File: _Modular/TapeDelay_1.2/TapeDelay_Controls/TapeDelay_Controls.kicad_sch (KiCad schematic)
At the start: 27 parts, among them J1 Interrupt, J3 Encoder/Enter/ESC, J4 OLED, J5 CPU I2C, SW1 Unload, SW2 Run/Pause, SW3 RotaryEncoder_Switch, SW4 Escape, U1 PCF8574

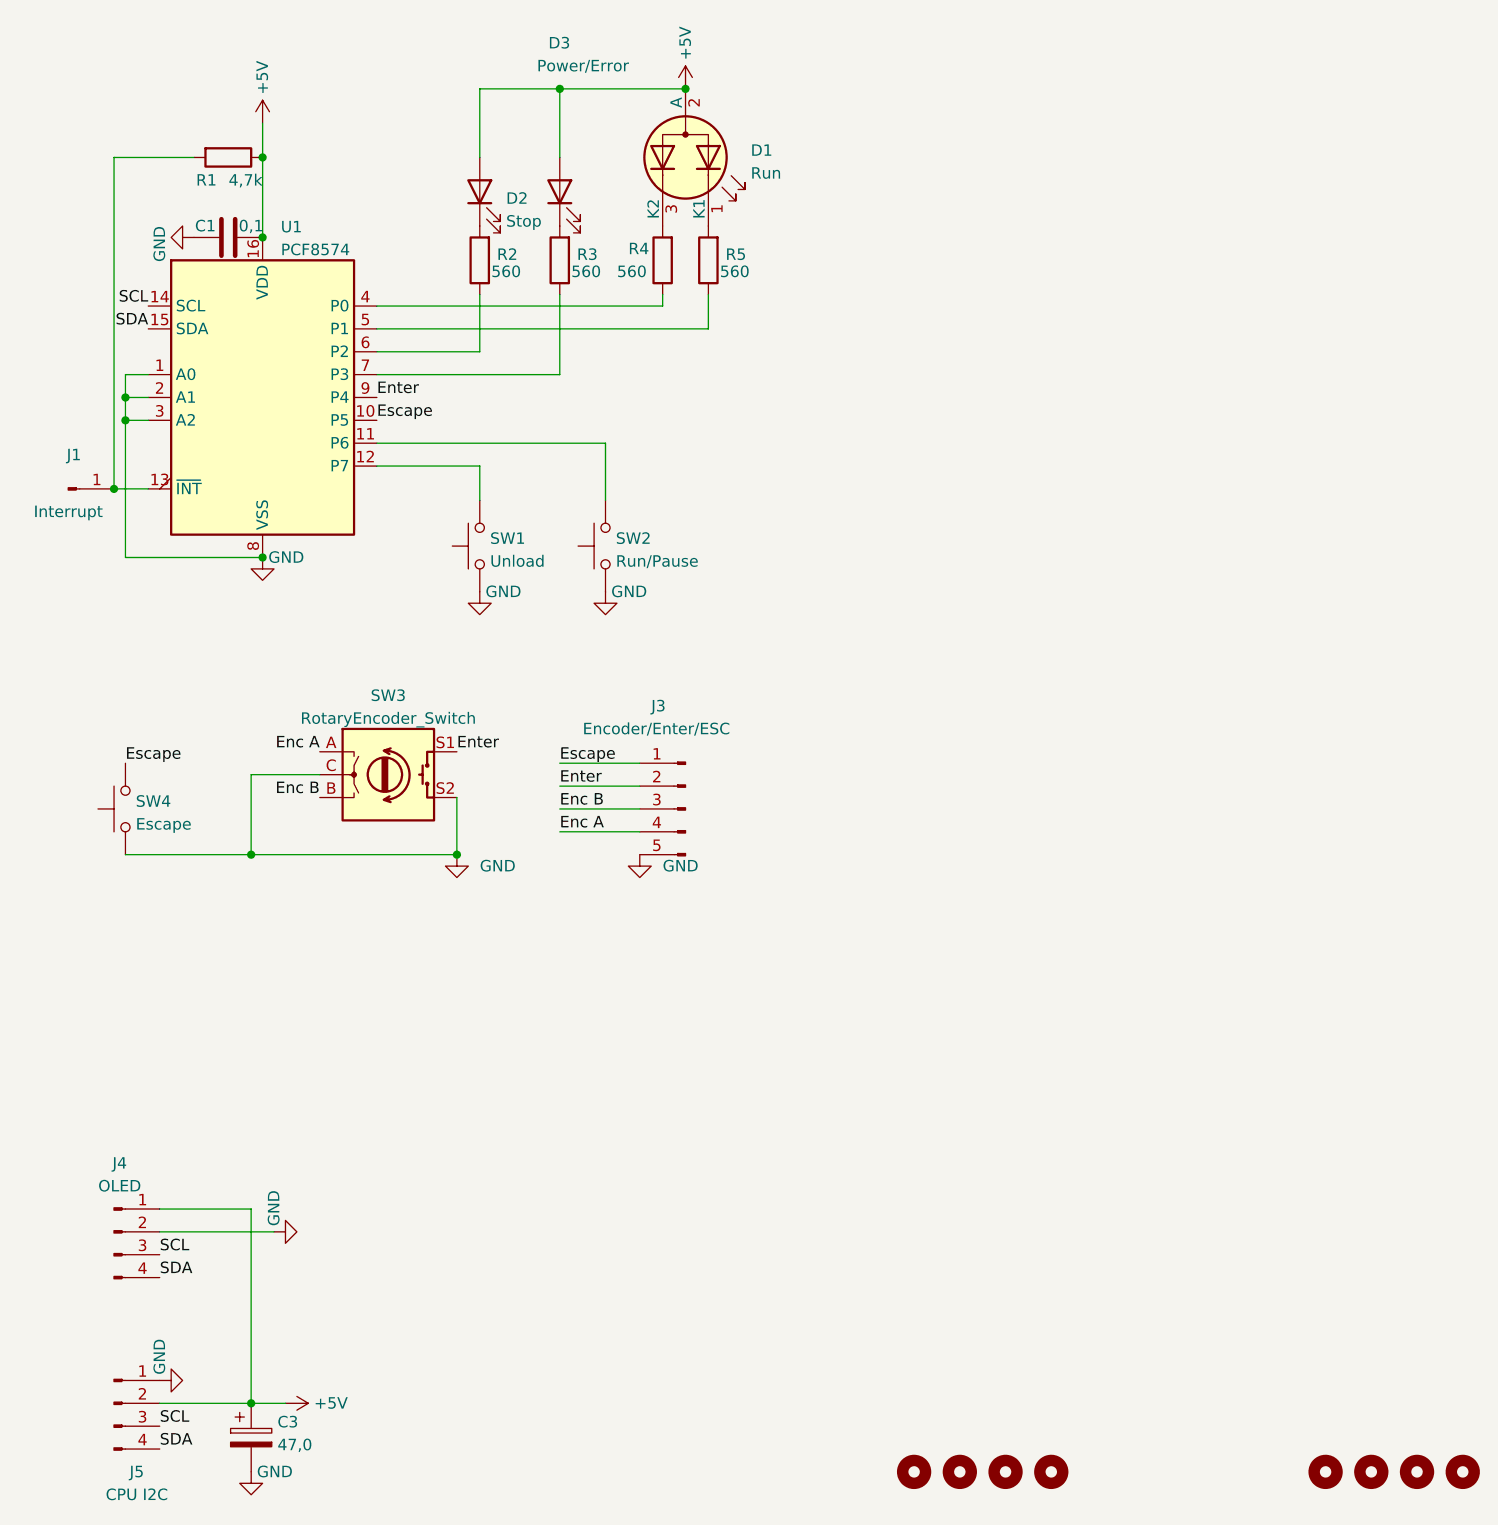
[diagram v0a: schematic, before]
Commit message: up
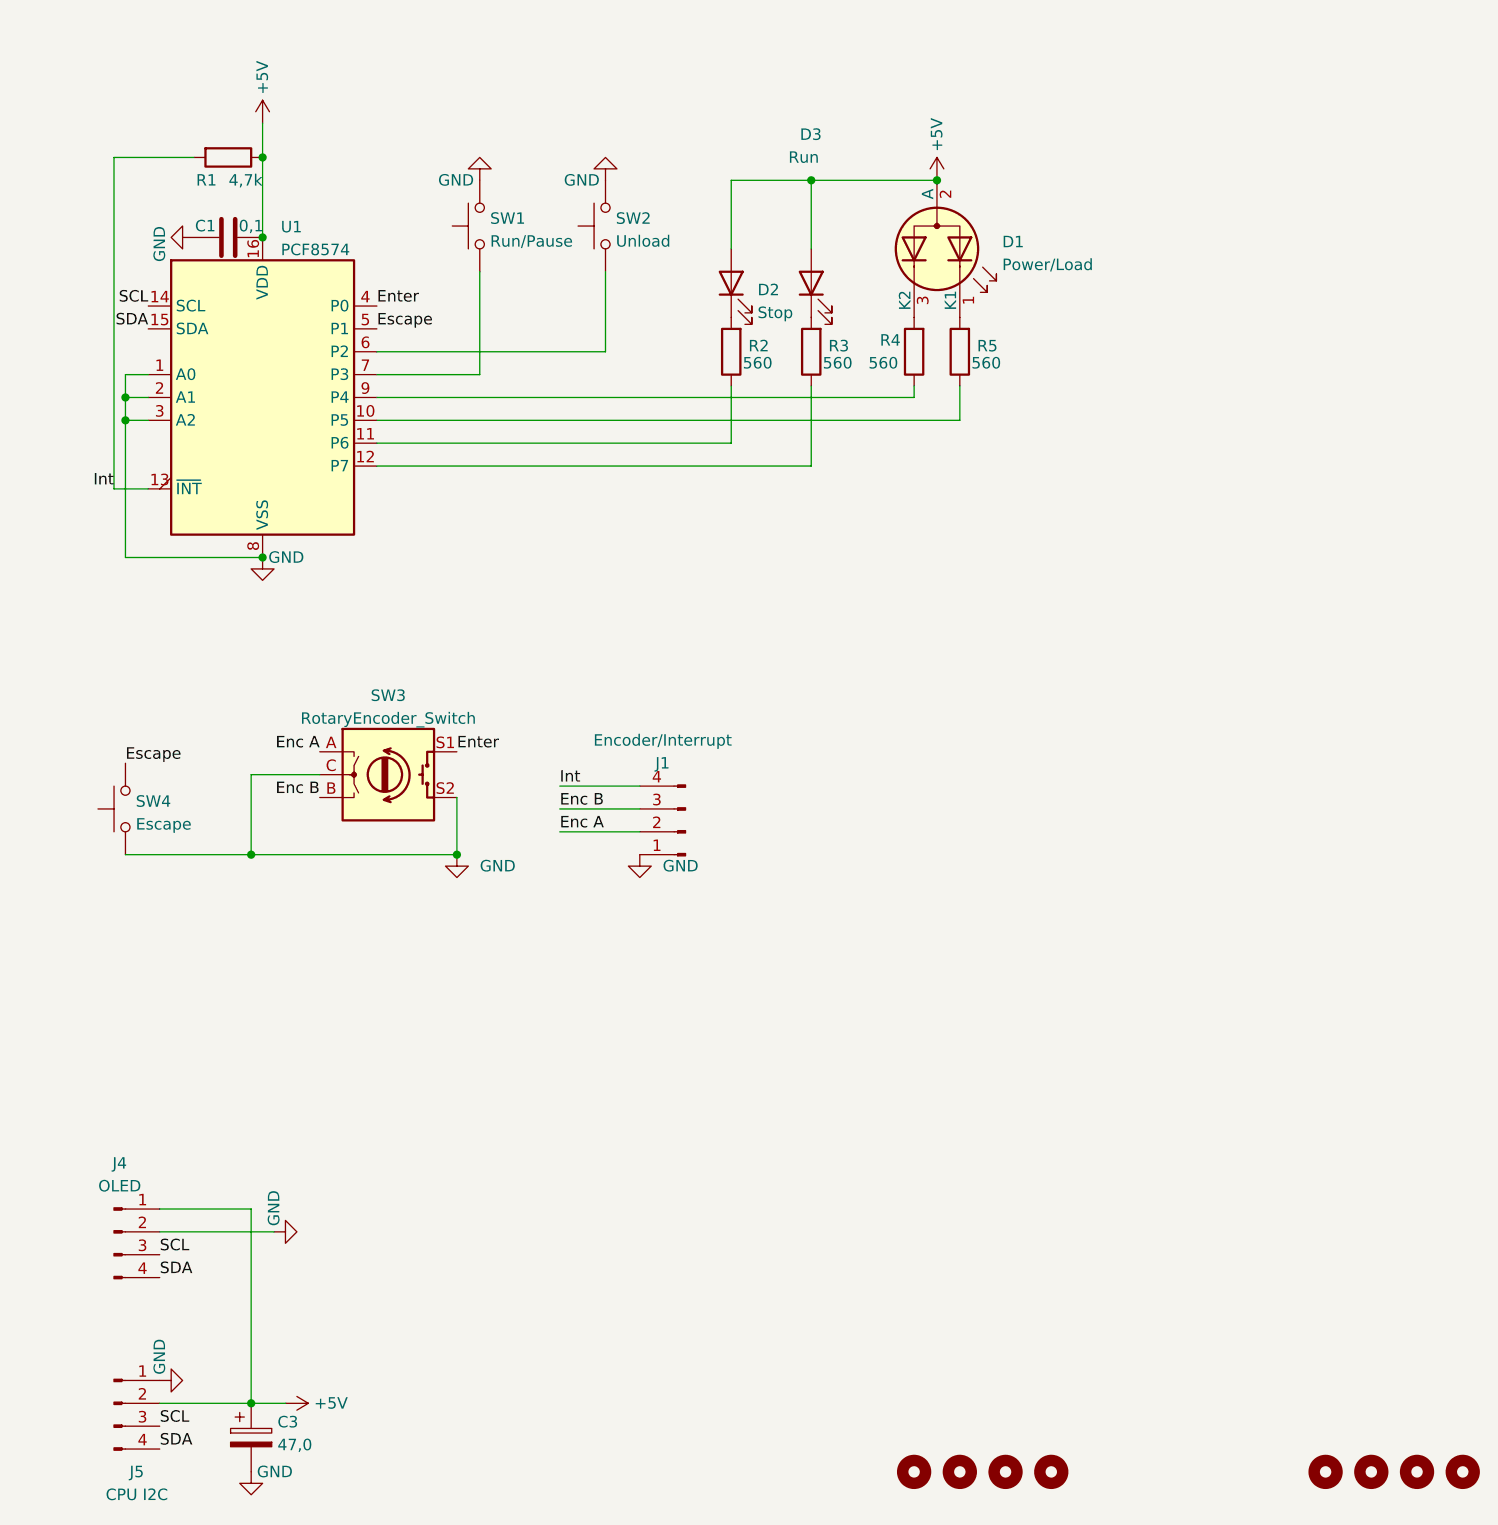
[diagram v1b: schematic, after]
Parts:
- removed J1: Interrupt, Connector_PinHeader_2.54mm:PinHeader_1x01_P2.54mm_Vertical, symbol Connector:Conn_01x01_Male
- removed J3: Encoder/Enter/ESC, Connector_PinHeader_2.54mm:PinHeader_1x05_P2.54mm_Vertical, symbol Connector:Conn_01x05_Male
- added J1: Encoder/Interrupt, Connector_PinHeader_2.54mm:PinHeader_1x04_P2.54mm_Vertical, symbol Connector:Conn_01x04_Male
- D1: value Run -> Power/Load
- D3: value Power/Error -> Run
- SW1: value Unload -> Run/Pause
- SW2: value Run/Pause -> Unload
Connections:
- net Enc A: now also J1.2 (Pin_2)
- net Enc B: now also J1.3 (Pin_3)
- net Enter: now also U1.4 (P0); no longer U1.9 (P4)
- net Escape: now also U1.5 (P1); no longer U1.10 (P5)
- net GND: now also J1.1 (Pin_1)
- net Int: now reaches R1.2, U1.13 (~{INT})
- net Int: now also J1.4 (Pin_4)
- net at R3.1: now also U1.12 (P7); no longer U1.7 (P3)
- net at R4.1: now also U1.9 (P4); no longer U1.4 (P0)
- net at SW1.2: now also U1.7 (P3); no longer U1.12 (P7)
- net at SW2.2: now also U1.6 (P2); no longer U1.11 (P6)
- net at R2.1: now also U1.11 (P6); no longer U1.6 (P2)
- net at R5.1: now also U1.10 (P5); no longer U1.5 (P1)
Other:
- moved on the sheet: D1, D2, D3, R2, R3, R4, R5, SW1, SW2

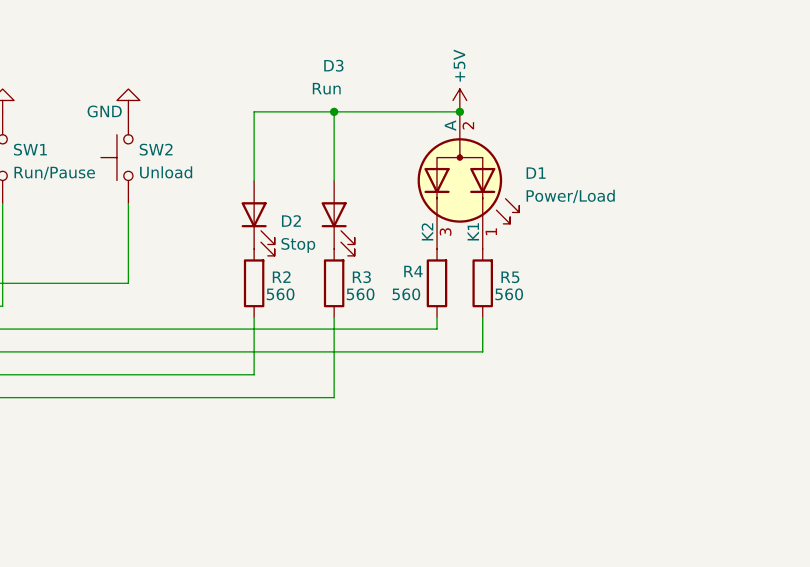
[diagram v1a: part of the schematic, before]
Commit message: up
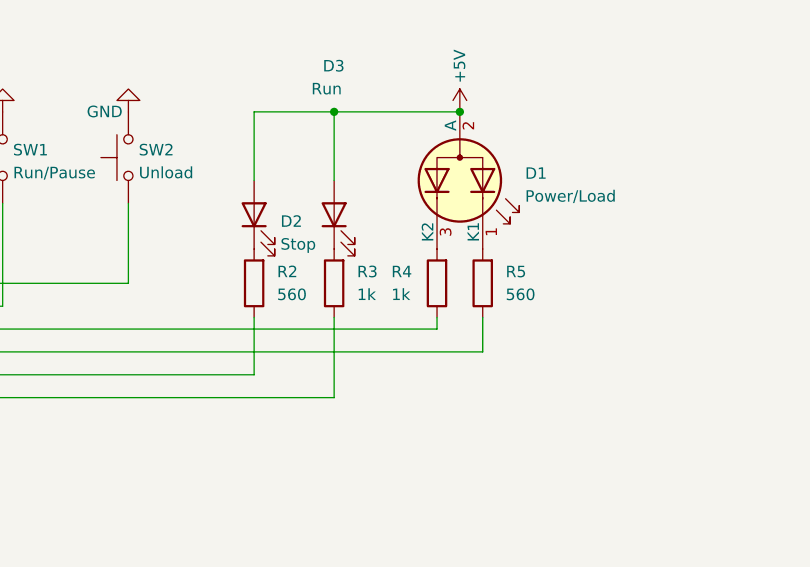
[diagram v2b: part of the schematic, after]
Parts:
- R3, R4: value 560 -> 1k
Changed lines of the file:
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@@
   (symbol (lib_id "Device:R") (at 99.06 67.31 180) (unit 1)
     (in_bom yes) (on_board yes)
-    (property "Reference" "R3" (id 0) (at 100.965 66.675 0)
-      (effects (font (size 1.27 1.27)) (justify right))
-    )
-    (property "Value" "560" (id 1) (at 100.33 68.58 0)
+    (property "Reference" "R3" (id 0) (at 101.6 66.04 0)
+      (effects (font (size 1.27 1.27)) (justify right))
+    )
+    (property "Value" "1k" (id 1) (at 101.6 68.58 0)
       (effects (font (size 1.27 1.27)) (justify right))
     )
@@
   (symbol (lib_id "Device:R") (at 110.49 67.31 180) (unit 1)
     (in_bom yes) (on_board yes)
-    (property "Reference" "R4" (id 0) (at 106.68 66.04 0)
-      (effects (font (size 1.27 1.27)) (justify right))
-    )
-    (property "Value" "560" (id 1) (at 105.41 68.58 0)
+    (property "Reference" "R4" (id 0) (at 105.41 66.04 0)
+      (effects (font (size 1.27 1.27)) (justify right))
+    )
+    (property "Value" "1k" (id 1) (at 105.41 68.58 0)
       (effects (font (size 1.27 1.27)) (justify right))
     )
@@
   (symbol (lib_id "Device:R") (at 90.17 67.31 180) (unit 1)
     (in_bom yes) (on_board yes)
-    (property "Reference" "R2" (id 0) (at 92.075 66.675 0)
-      (effects (font (size 1.27 1.27)) (justify right))
-    )
-    (property "Value" "560" (id 1) (at 91.44 68.58 0)
+    (property "Reference" "R2" (id 0) (at 92.71 66.04 0)
+      (effects (font (size 1.27 1.27)) (justify right))
+    )
+    (property "Value" "560" (id 1) (at 92.71 68.58 0)
       (effects (font (size 1.27 1.27)) (justify right))
     )
@@
   (symbol (lib_id "Device:R") (at 115.57 67.31 180) (unit 1)
     (in_bom yes) (on_board yes)
-    (property "Reference" "R5" (id 0) (at 117.475 66.675 0)
-      (effects (font (size 1.27 1.27)) (justify right))
-    )
-    (property "Value" "560" (id 1) (at 116.84 68.58 0)
+    (property "Reference" "R5" (id 0) (at 118.11 66.04 0)
+      (effects (font (size 1.27 1.27)) (justify right))
+    )
+    (property "Value" "560" (id 1) (at 118.11 68.58 0)
       (effects (font (size 1.27 1.27)) (justify right))
     )
@@
     )
     (path "/371bfc8a-7519-47d9-a97b-f1790b89b089"
-      (reference "R3") (unit 1) (value "560") (footprint "Resistor_SMD:R_1206_3216Metric_Pad1.30x1.75mm_HandSolder")
+      (reference "R3") (unit 1) (value "1k") (footprint "Resistor_SMD:R_1206_3216Metric_Pad1.30x1.75mm_HandSolder")
     )
     (path "/3ec11503-a035-46af-a935-fa778f39979c"
-      (reference "R4") (unit 1) (value "560") (footprint "Resistor_SMD:R_1206_3216Metric_Pad1.30x1.75mm_HandSolder")
+      (reference "R4") (unit 1) (value "1k") (footprint "Resistor_SMD:R_1206_3216Metric_Pad1.30x1.75mm_HandSolder")
     )
     (path "/c870de65-a296-4353-94af-1a3965a29084"
